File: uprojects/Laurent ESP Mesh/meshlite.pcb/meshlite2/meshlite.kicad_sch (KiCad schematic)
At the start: 18 parts, among them J1 DCJ200-10-A-XX-K_REVA, J2 B5PS-VH, J3 B5PS-VH, K2 FINDER-36.11, Q1 MMBT2222A, U1 MOUDLE-SEEEDUINO-XIAO-ESP32C3, U2 INA219, U3 YAAJ_DCDC_StepDown_LM2596

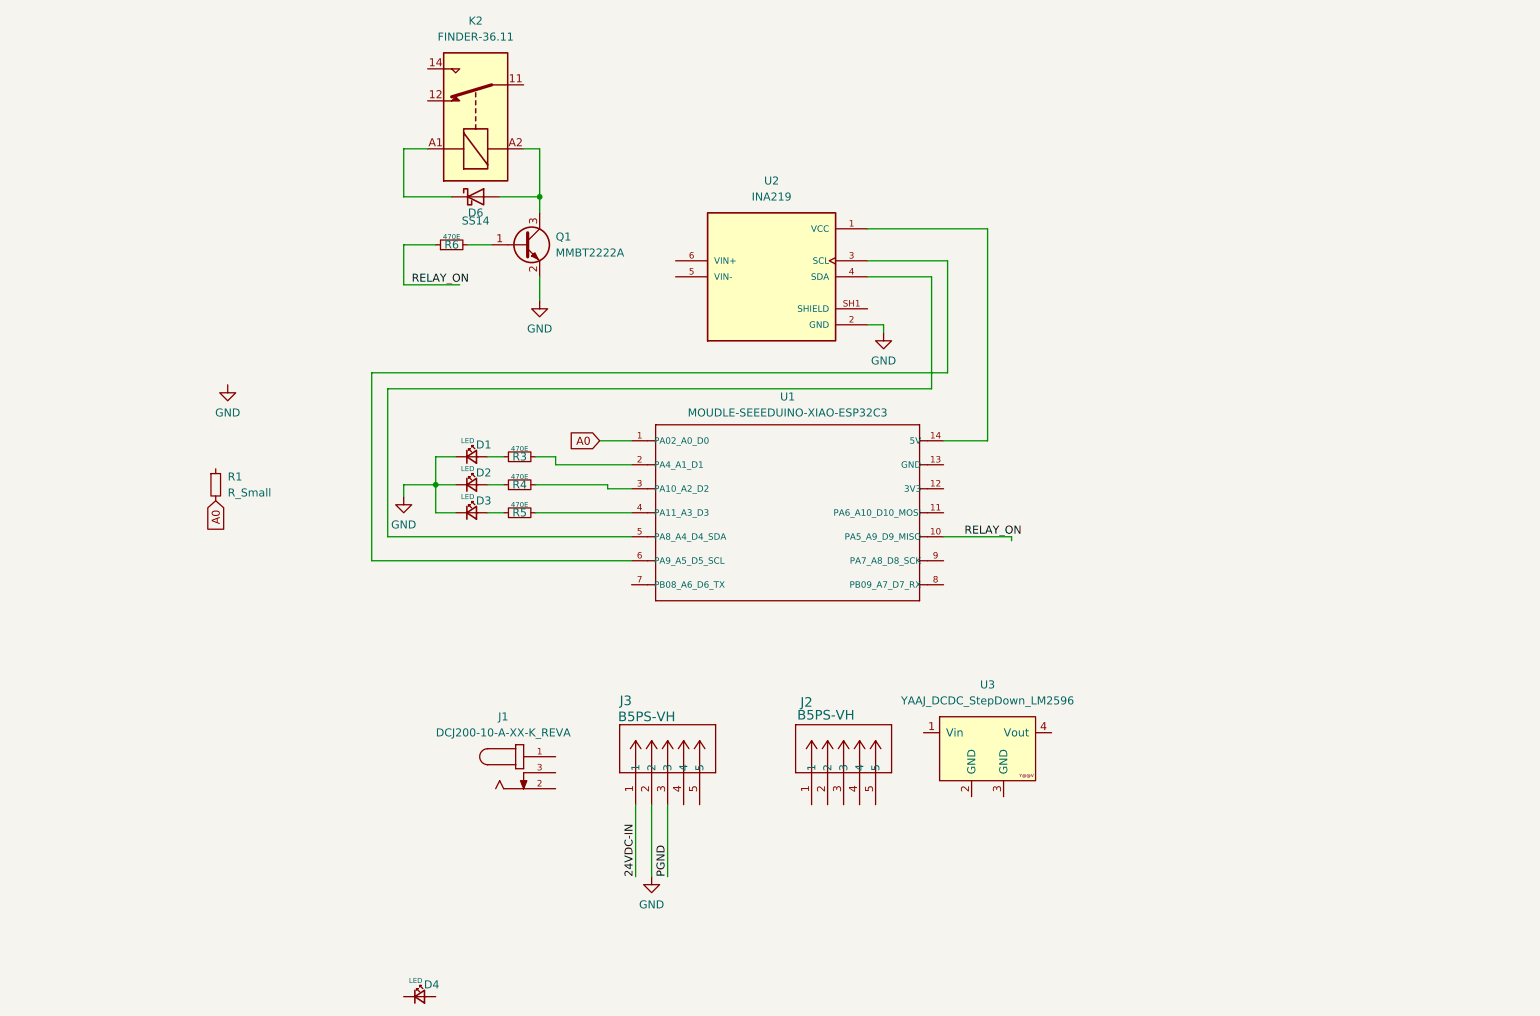
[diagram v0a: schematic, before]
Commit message: Update 23 Feb 2026
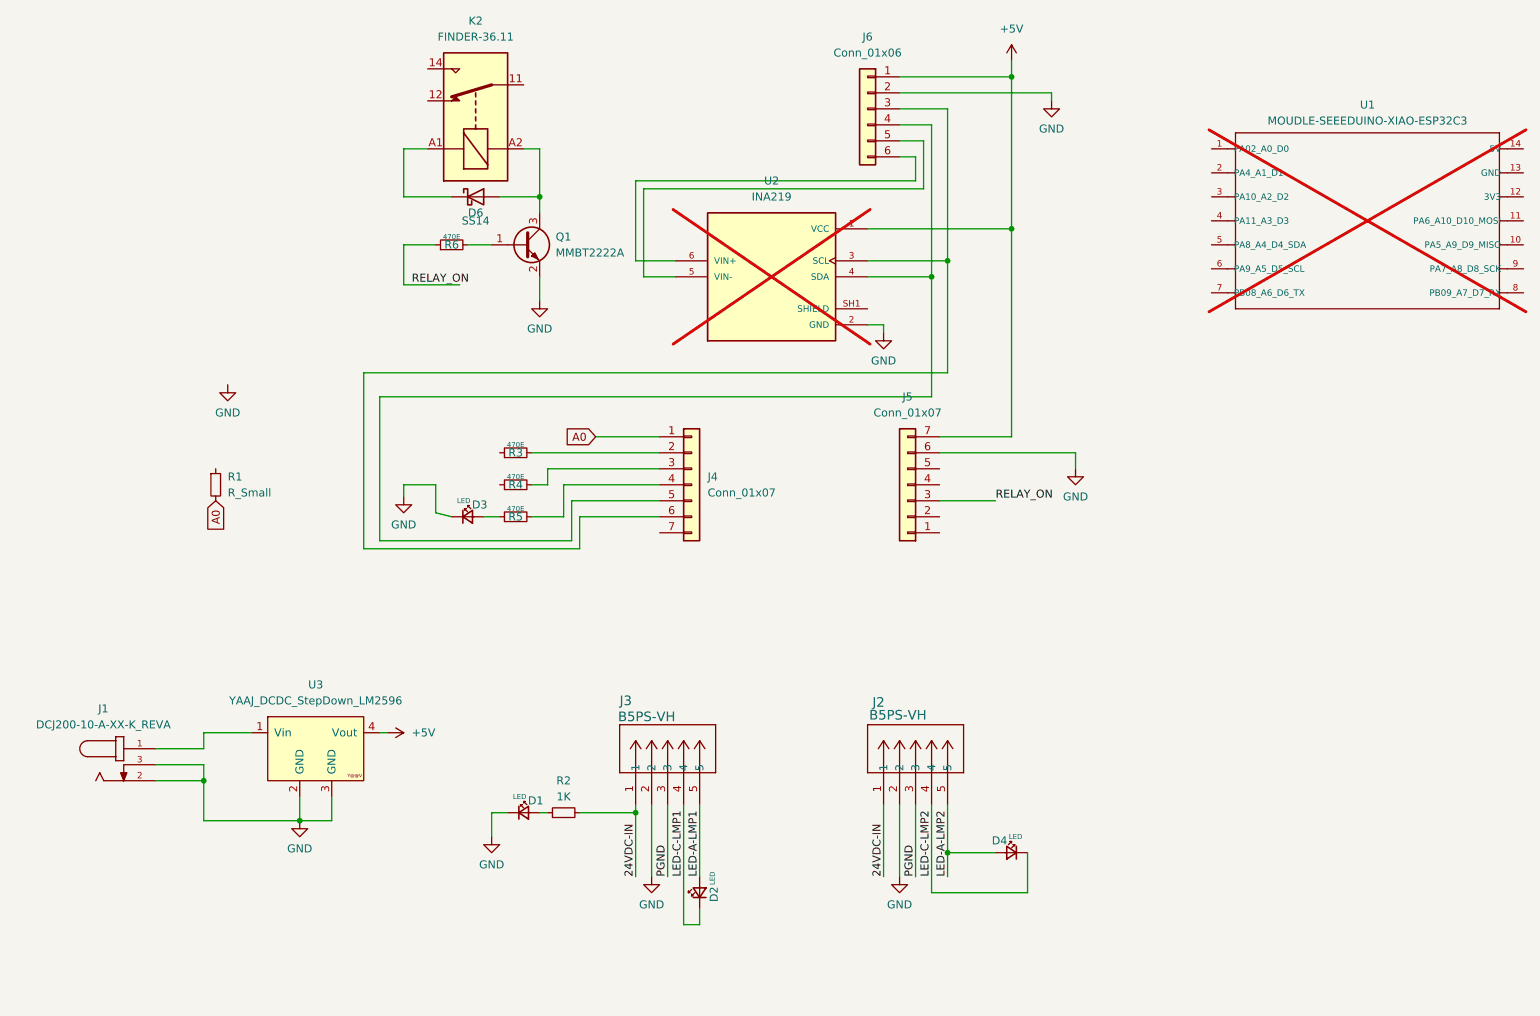
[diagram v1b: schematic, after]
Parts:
- added J4, J5: Conn_01x07, Connector_PinSocket_2.54mm:PinSocket_1x07_P2.54mm_Vertical, symbol Connector_Generic:Conn_01x07
- added J6: Conn_01x06, Connector_PinSocket_2.54mm:PinSocket_1x06_P2.54mm_Vertical, symbol Connector_Generic:Conn_01x06
- added R2: 1K, Resistor_SMD:R_0603_1608Metric, symbol Device:R_Small
- U1, U2: now not fitted; now left out of the parts list
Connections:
- net 24VDC-IN: now also J2.1, R2.2
- net A0: now also J4.1 (Pin_1); no longer U1.1 (PA02_A0_D0)
- net GND: now also J1.2, J1.3, J2.2, U3.2 (GND), U3.3 (GND), J5.6 (Pin_6), J6.2 (Pin_2); no longer D2.1 (K)
- net PGND: now also J2.3
- net RELAY_ON: now also J5.3 (Pin_3); no longer U1.10 (PA5_A9_D9_MISO)
- net at R3.1: no longer D1.2 (A)
- net at R3.2: now also J4.2 (Pin_2); no longer U1.2 (PA4_A1_D1)
- net at R5.2: now also J4.4 (Pin_4); no longer U1.4 (PA11_A3_D3)
- net at U1.14 (5V): no longer U2.1 (VCC)
- net at U2.3 (SCL): now also J4.6 (Pin_6), J6.3 (Pin_3); no longer U1.6 (PA9_A5_D5_SCL)
- net at U2.4 (SDA): now also J4.5 (Pin_5), J6.4 (Pin_4); no longer U1.5 (PA8_A4_D4_SDA)
- net at U2.5 (VIN-), U2.VIN-: now also J6.5 (Pin_5)
- net at U2.6 (VIN+), U2.VIN+: now also J6.6 (Pin_6)
- net at R4.1: no longer D2.2 (A)
- net LED-C-LMP2: now reaches J2.4
- net LED-C-LMP2: now also D4.1 (K)
- net LED-A-LMP2: now reaches J2.5
- net LED-A-LMP2: now also D4.2 (A)
- net at J1.1: now also U3.1 (Vin)
- net LED-C-LMP1: now reaches J3.4
- net LED-C-LMP1: now also D2.1 (K)
- net LED-A-LMP1: now reaches J3.5
- net LED-A-LMP1: now also D2.2 (A)
- net at R4.2: now also J4.3 (Pin_3); no longer U1.3 (PA10_A2_D2)
- net +5V: now reaches U3.4 (Vout)
- net +5V: now also U2.1 (VCC), J5.7 (Pin_7), J6.1 (Pin_1)
- new net: D1.2 (A), R2.1
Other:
- moved on the sheet: D1, D2, D3, D4, J1, J2, R3, R4, R5, U3
